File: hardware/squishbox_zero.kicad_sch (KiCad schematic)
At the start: 18 parts, among them J1 AudioJack4_SwitchTR1, J3 LED, J4 UART_HDR, J5 USB_A, U1 XC6206P332MR-G, U2 PCM5102A

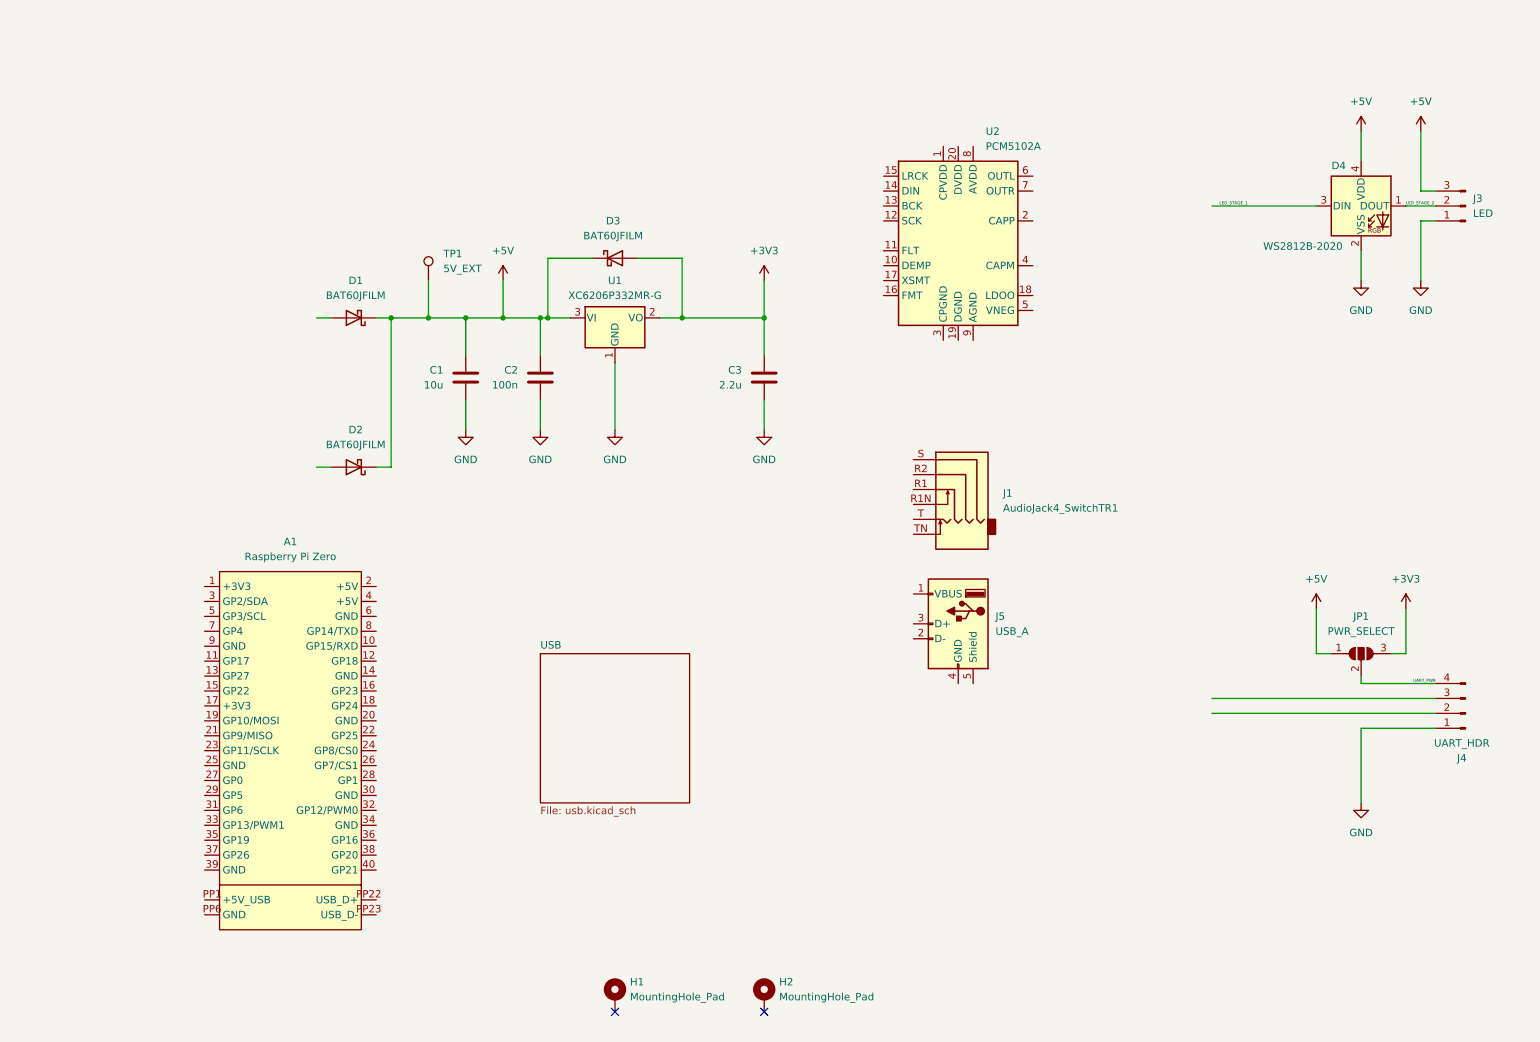
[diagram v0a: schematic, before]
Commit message: Audio circuit layout
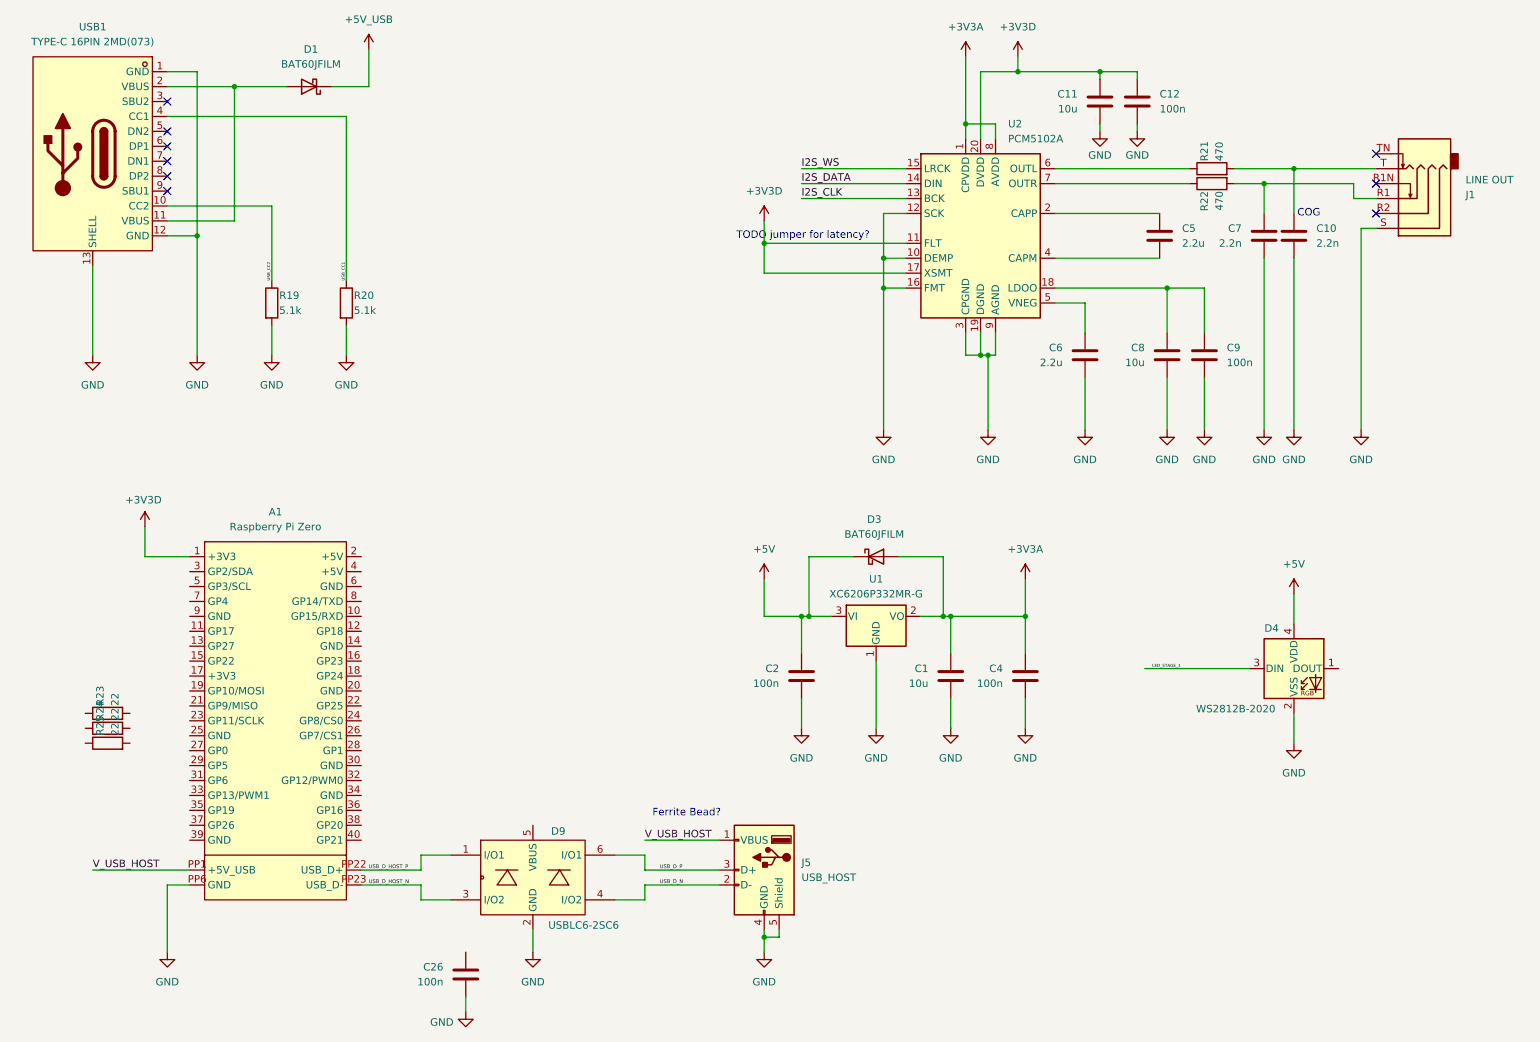
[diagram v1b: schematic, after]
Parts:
- removed C3: 2.2u, Capacitor_SMD:C_0402_1005Metric, symbol Device:C
- removed D2: BAT60JFILM, Diode_SMD:D_SOD-323, symbol Device:D_Schottky
- removed H1, H2: MountingHole_Pad, MountingHole:MountingHole_3.2mm_M3_Pad, symbol Mechanical:MountingHole_Pad
- removed J3: LED, Connector_PinHeader_1.27mm:PinHeader_1x03_P1.27mm_Vertical, symbol Connector:Conn_01x03_Pin
- removed J4: UART_HDR, Connector_PinHeader_2.54mm:PinHeader_1x04_P2.54mm_Horizontal, symbol Connector:Conn_01x04_Pin
- removed JP1: PWR_SELECT, Jumper:SolderJumper-3_P1.3mm_Open_RoundedPad1.0x1.5mm_NumberLabels, symbol Jumper:SolderJumper_3_Open
- removed TP1: 5V_EXT, TestPoint:TestPoint_Pad_D1.5mm, symbol Connector:TestPoint
- added C10, C7: 2.2n, Capacitor_SMD:C_0402_1005Metric, symbol Device:C
- added C11, C8: 10u, Capacitor_SMD:C_0603_1608Metric, symbol Device:C
- added C12, C26, C4, C9: 100n, Capacitor_SMD:C_0402_1005Metric, symbol Device:C
- added C5, C6: 2.2u, Capacitor_SMD:C_0402_1005Metric, symbol Device:C
- added D9: USBLC6-2SC6, _lib:SOT-23-6_L2.9-W1.6-P0.95-LS2.8-BL, symbol _lib:USBLC6-2SC6
- added R19, R20: 5.1k, Resistor_SMD:R_0402_1005Metric, symbol Device:R
- added R21, R22: 470, Resistor_SMD:R_0402_1005Metric, symbol Device:R
- added R23, R24, R25: 22, Resistor_SMD:R_0402_1005Metric, symbol Device:R
- added USB1: TYPE-C 16PIN 2MD(073), _lib:USB-C-SMD_TYPE-C-16PIN, symbol _lib:USB-C-SMD_TYPE-C-16PIN
- J1: value AudioJack4_SwitchTR1 -> LINE OUT
- J5: value USB_A -> USB_HOST
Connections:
- net +3V3 is gone; now on net +3V3A: D3.2 (A), U1.2 (VO)
- net +5V: no longer C1.1, D1.1 (K)
- net GND: now also A1.PP6 (GND), J1.S, J5.4 (GND), J5.5 (Shield), U2.10 (DEMP), U2.12 (SCK), U2.16 (FMT), U2.19 (DGND), U2.3 (CPGND), U2.9 (AGND), C10.2, C11.2, C12.2, C26.2, C4.2, C6.2, C7.2, C8.2, C9.2, D9.2 (GND), R19.2, R20.2, USB1.1 (GND), USB1.12 (GND), USB1.13 (SHELL)
- net V_USB_HOST: now reaches J5.1 (VBUS)
- net V_USB_HOST: now also A1.PP1 (+5V_USB)
- net USB_D_N: now reaches J5.2 (D-)
- net USB_D_N: now also D9.4 (I/O2)
- net USB_D_P: now reaches J5.3 (D+)
- net USB_D_P: now also D9.6 (I/O1)
- net at D1.2 (A): now also USB1.11 (VBUS), USB1.2 (VBUS)
- net at J1.R1: now also C7.1, R22.2
- net at J1.T: now also C10.1, R21.2
- net +3V3A: now reaches U2.1 (CPVDD)
- net +3V3A: now also C1.1, U2.8 (AVDD), C4.1
- net +3V3D: now reaches U2.11 (FLT)
- net +3V3D: now also A1.1 (+3V3), U2.17 (XSMT), U2.20 (DVDD), C11.1, C12.1
- net I2S_CLK: now reaches U2.13 (BCK)
- net I2S_DATA: now reaches U2.14 (DIN)
- net I2S_WS: now reaches U2.15 (LRCK)
- net at U2.18 (LDOO): now also C8.1, C9.1
- net at U2.2 (CAPP): now also C5.1
- net at U2.4 (CAPM): now also C5.2
- net at U2.5 (VNEG): now also C6.1
- net at U2.6 (OUTL): now also R21.1
- net at U2.7 (OUTR): now also R22.1
- net USB_D_HOST_P: now reaches A1.PP22 (USB_D+)
- net USB_D_HOST_P: now also D9.1 (I/O1)
- net USB_D_HOST_N: now reaches A1.PP23 (USB_D-)
- net USB_D_HOST_N: now also D9.3 (I/O2)
- net LED_STAGE_2: no longer names the net of D4.1 (DOUT)
- new net +5V_USB: D1.1 (K)
- new net USB_CC1: R20.1, USB1.4 (CC1)
- new net USB_CC2: R19.1, USB1.10 (CC2)
- no-connect marks 2 -> 9
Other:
- removed sheet USB
- note added: "COG"
- note added: "Ferrite Bead?"
- note added: "TODO jumper for latency?"
- moved on the sheet: A1, C1, C2, D1, D3, D4, J1, J5, U1, U2
